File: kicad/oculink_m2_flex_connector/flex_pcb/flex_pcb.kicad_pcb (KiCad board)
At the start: 2 copper layers, 29.7 x 17.8 mm, 2 parts, among them J1 Conn_01x38_Pin, J2 Conn_01x38_Pin

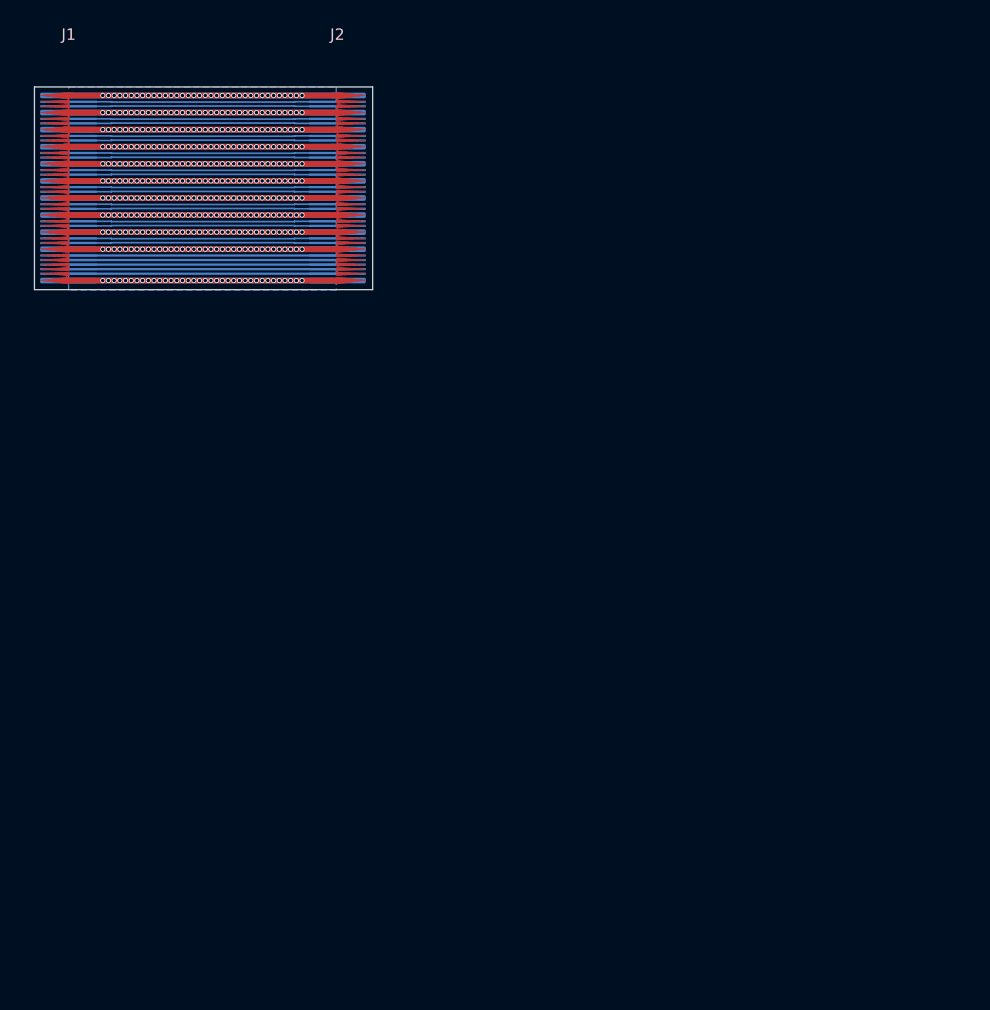
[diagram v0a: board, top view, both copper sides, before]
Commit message: Initial design and layout for flex pcb
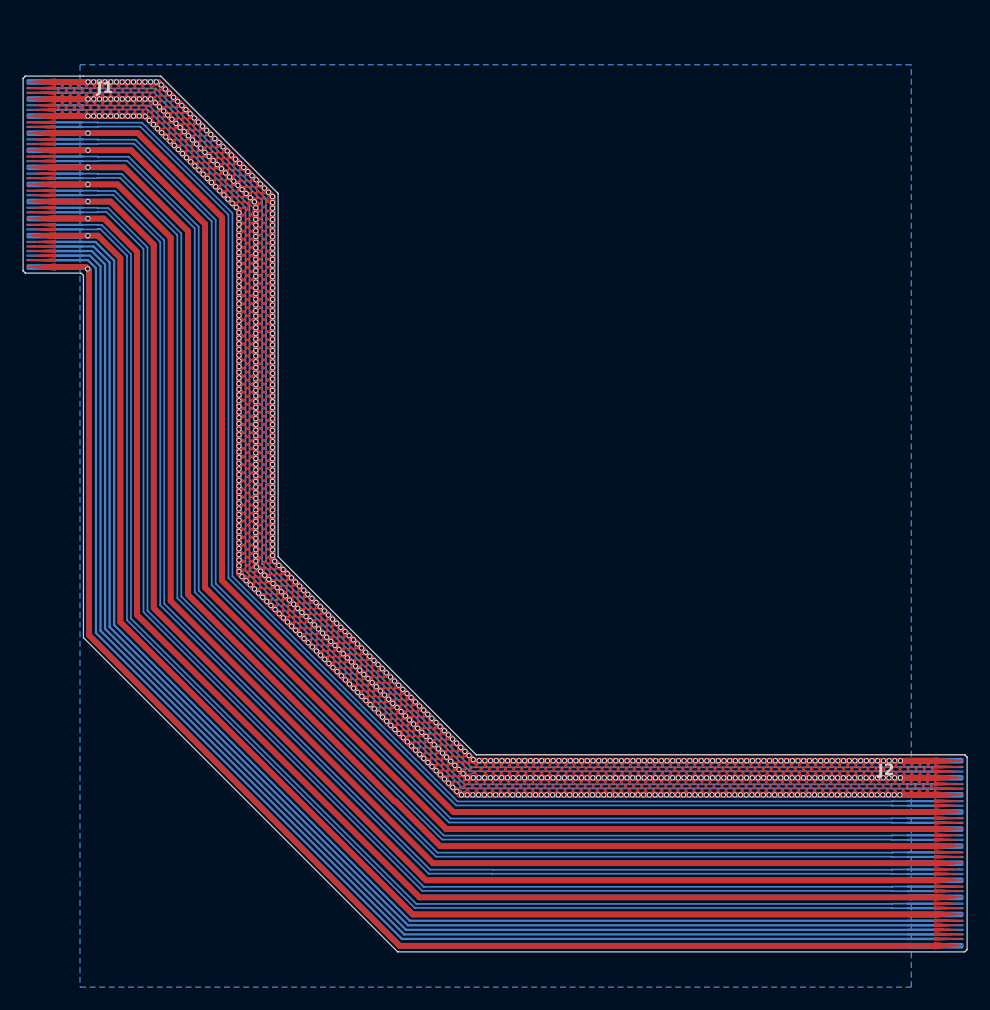
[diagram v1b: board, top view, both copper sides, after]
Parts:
- moved J2 78.5 mm to (170.1, 125.3)
- moved J1 1.69 mm to (92.8, 65.7)
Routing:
- net GND: track 517.7 -> 2654.9 mm, vias 396 -> 692
- net 3.3V_OPT: track 23.6 -> 120.7 mm
- net PERST: track 23.6 -> 120.7 mm
- net PEWAKE: track 23.6 -> 120.7 mm
- net PEDET: track 23.6 -> 120.7 mm
- net RX3-: track 23.6 -> 120.7 mm
- net CLKREQ: track 23.6 -> 120.7 mm
- net RX3+: track 23.6 -> 120.7 mm
- net TX1+: track 23.6 -> 120.7 mm
- net RX1-: track 23.6 -> 120.7 mm
- net TX1-: track 23.6 -> 120.7 mm
- net RX1+: track 23.6 -> 120.7 mm
- net TX0-: track 23.6 -> 120.7 mm
- net TX0+: track 23.6 -> 120.7 mm
- net RX2+: track 23.6 -> 120.7 mm
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- removed copper zone on F.Cu, net GND
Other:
- board size 29.7 x 17.8 mm -> 82.9 x 76.9 mm

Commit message: Finished initial layout of hatched plane for differential traces
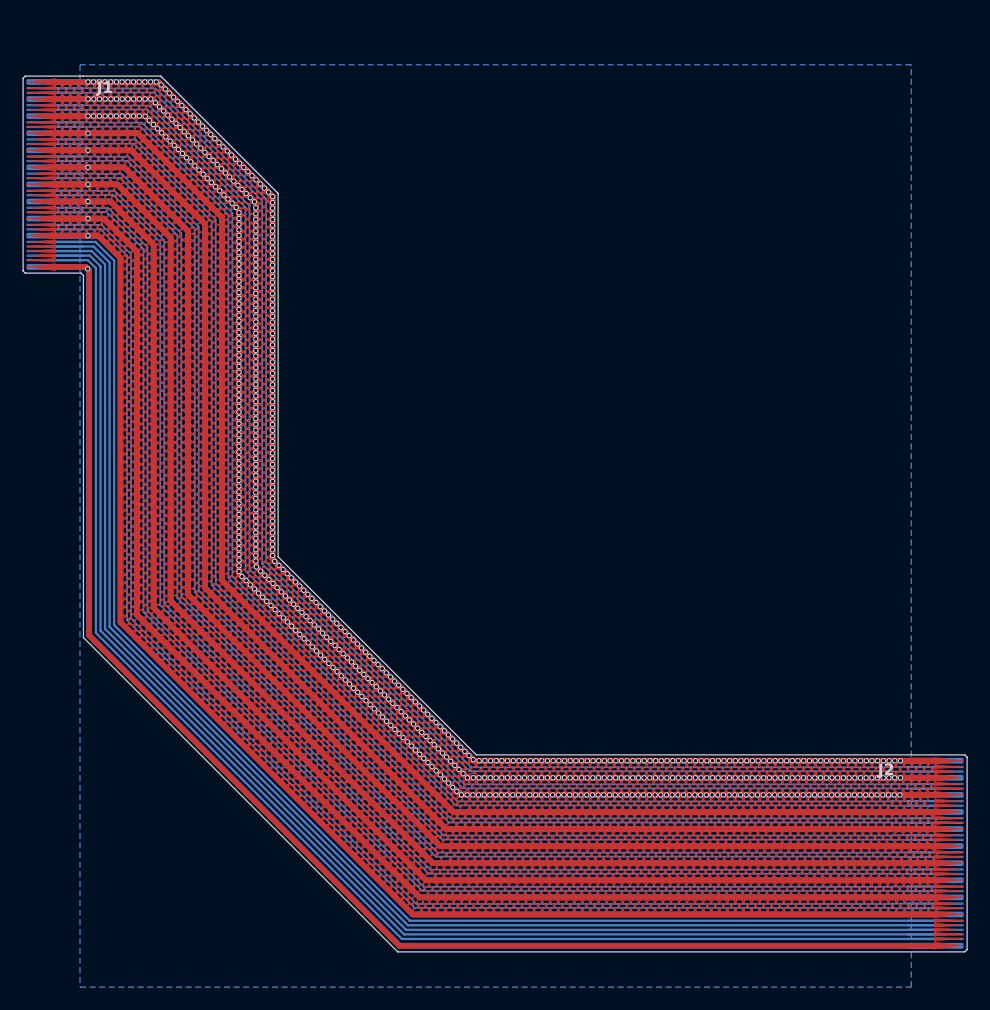
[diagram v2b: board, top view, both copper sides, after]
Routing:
- added copper zone on F.Cu, net GND
